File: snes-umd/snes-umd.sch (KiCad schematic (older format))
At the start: 1 part

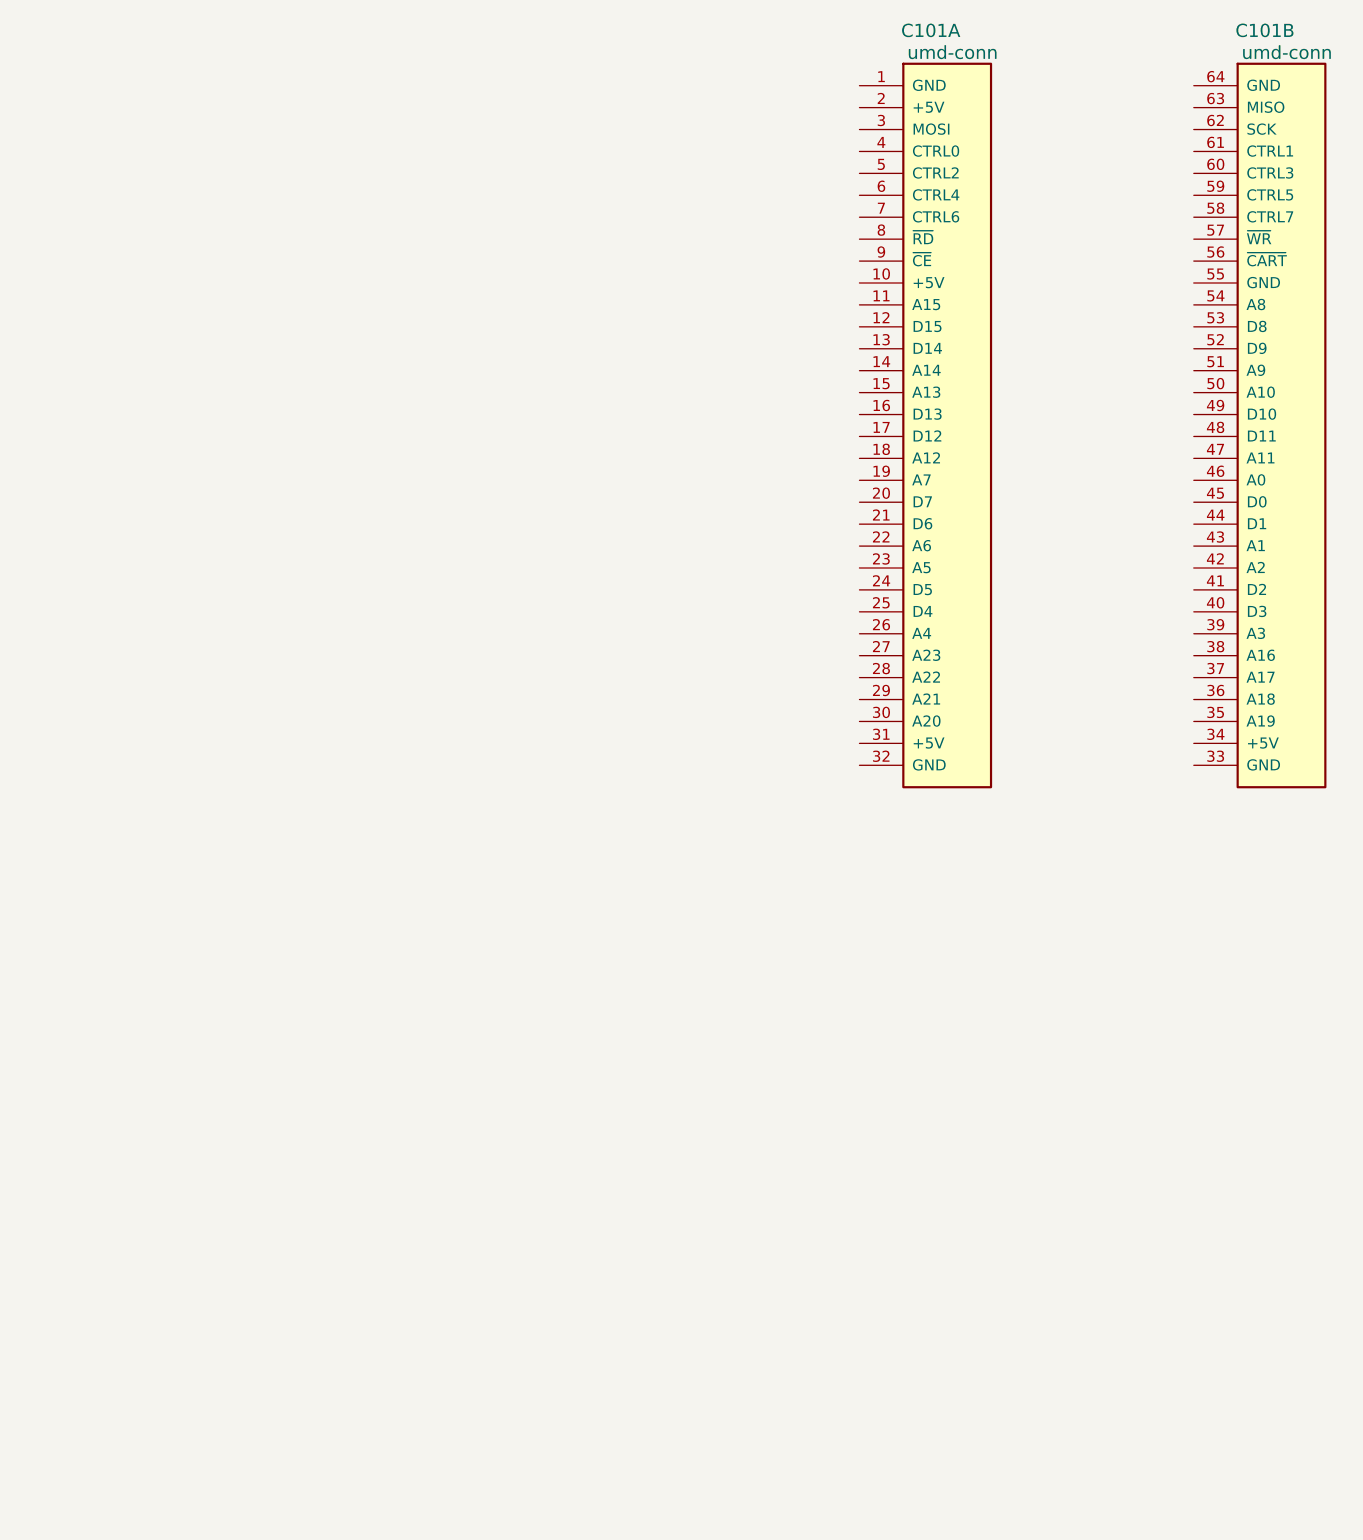
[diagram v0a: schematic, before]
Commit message: sch work on SNES adapter
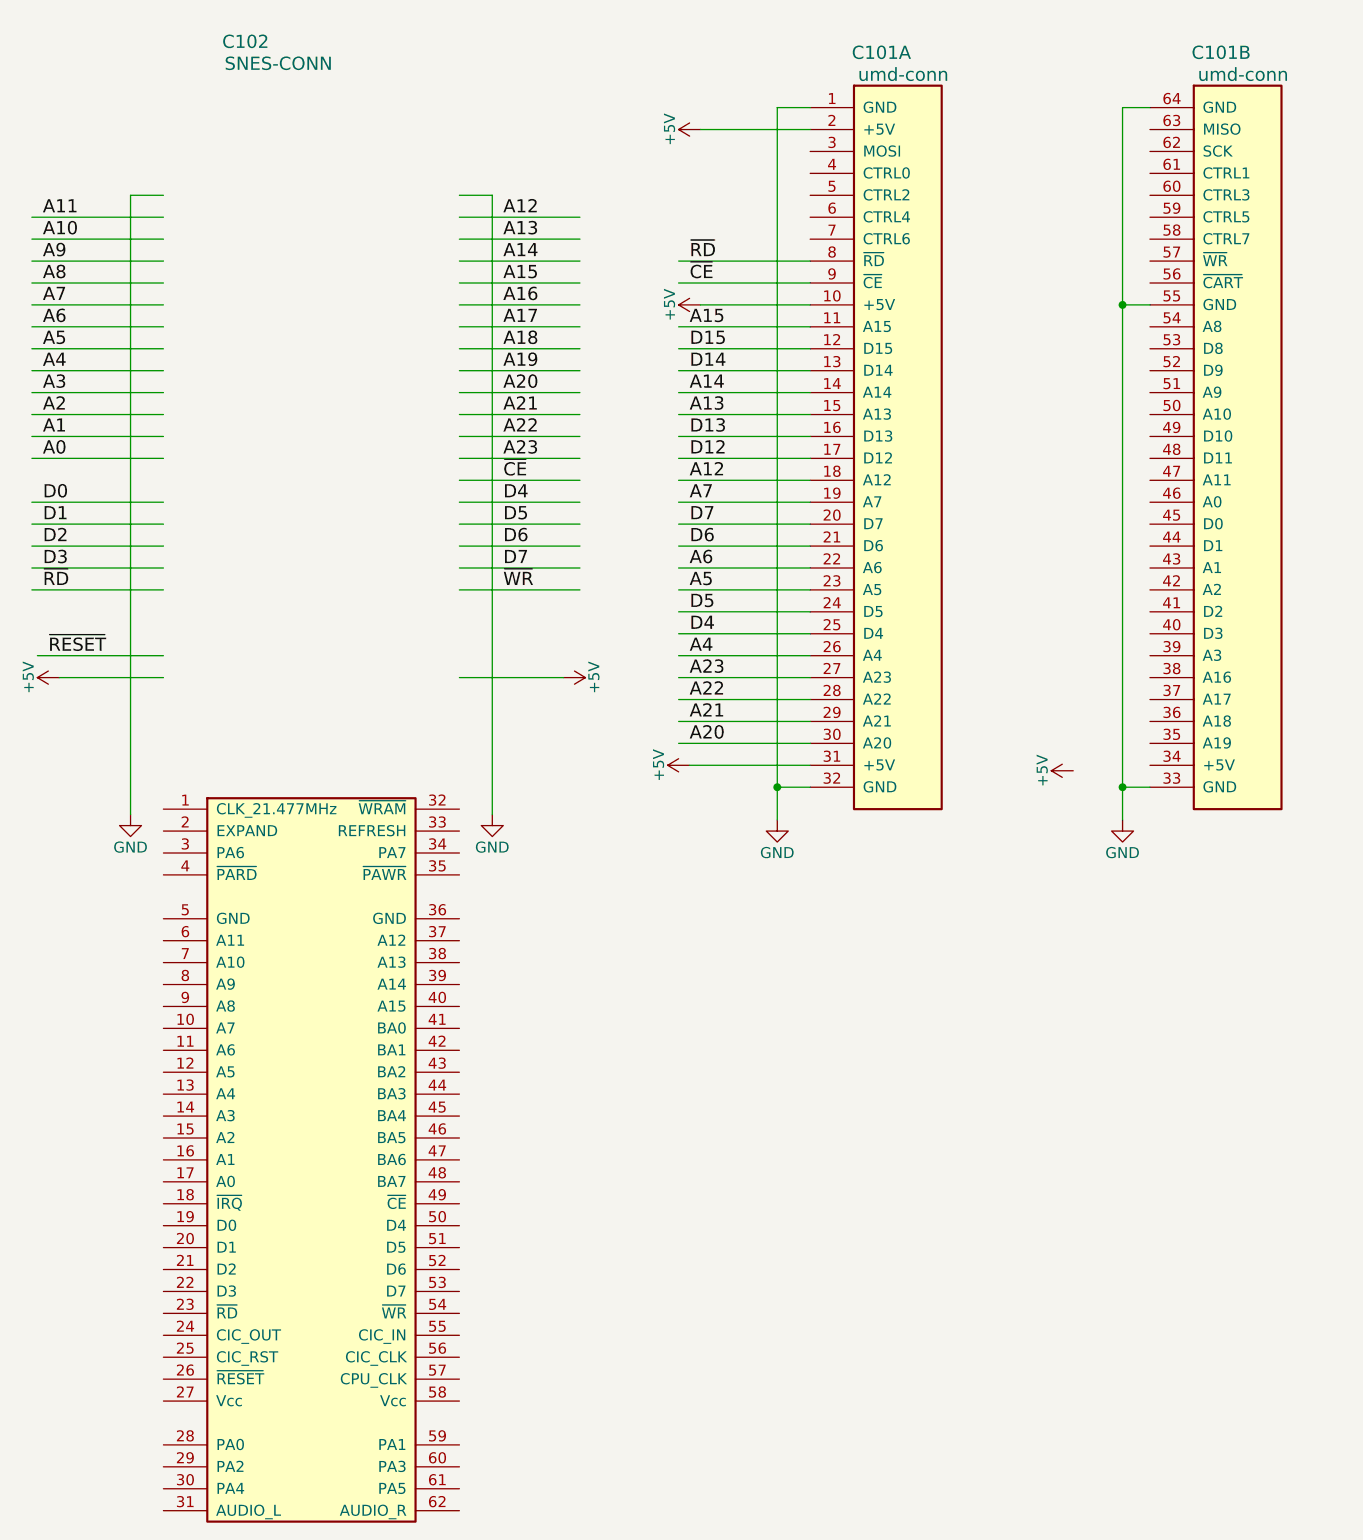
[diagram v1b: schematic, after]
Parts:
- added C102: SNES-CONN, db-thparts:SNES-CONN-EXP, symbol SNES-CONN
- C101: footprint (none) -> db-thparts:UMD-CONN-DIP64
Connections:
- net labels added: +5V, A0, A1, A10, A11, A12, A13, A14, A15, A16, A17, A18, A19, A2, A20, A21, A22, A23, A3, A4, A5, A6, A7, A8, A9, D0, D1, D12, D13, D14, D15, D2, D3, D4, D5, D6, D7, GND, ~CE, ~RD, ~RESET, ~WR
- wire segments 0 -> 74
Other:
- moved on the sheet: C101A, C101B
